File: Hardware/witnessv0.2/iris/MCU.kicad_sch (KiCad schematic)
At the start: 26 parts, among them J1 Conn_01x02, J4 Conn_01x02, U4 MCP23008-xML, U7 ESP32-C3FH4, Y1 F322540MUBCE2O

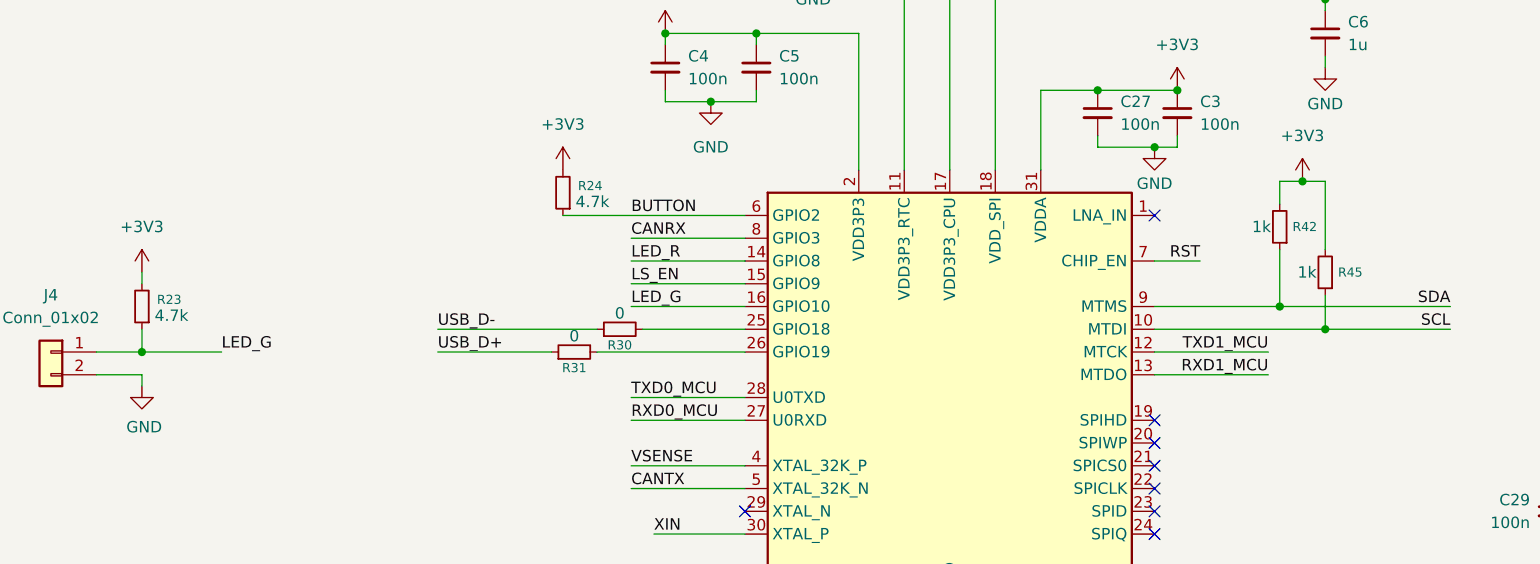
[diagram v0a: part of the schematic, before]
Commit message: iris release
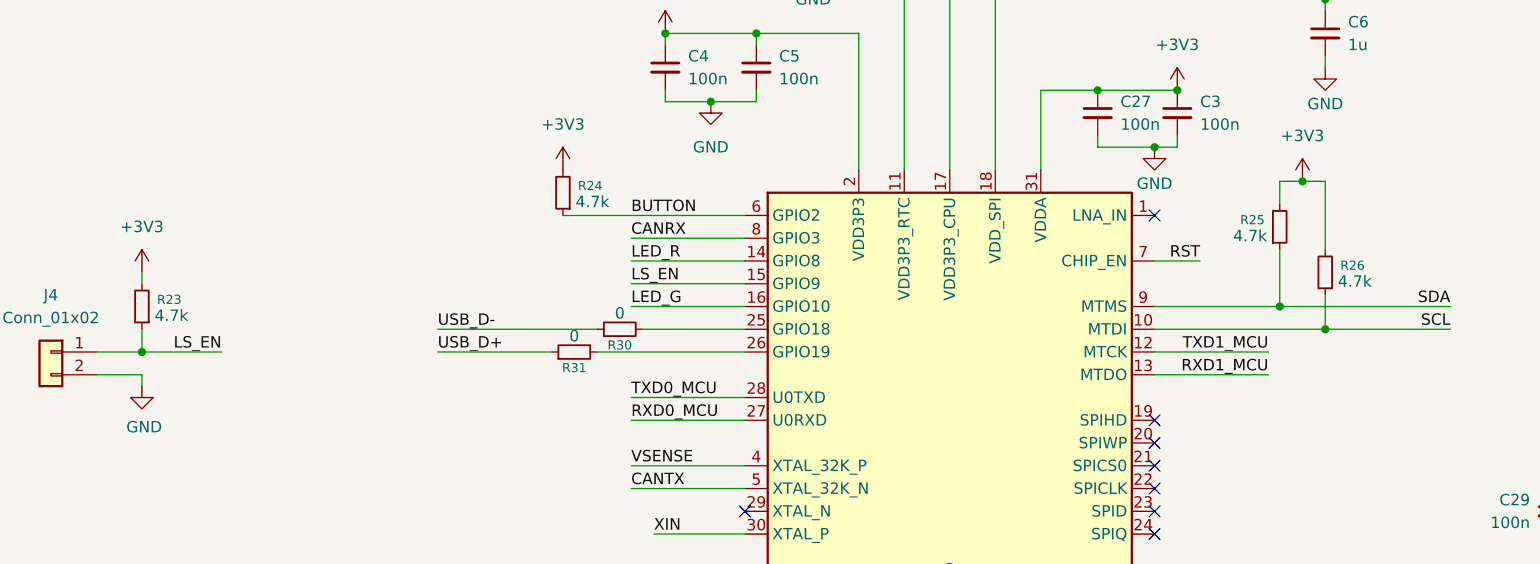
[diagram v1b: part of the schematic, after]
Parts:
- removed R42, R45: 1k, Resistor_SMD:R_0402_1005Metric, symbol Device:R_Small
- added R25, R26: 4.7k, Resistor_SMD:R_0402_1005Metric, symbol Device:R_Small
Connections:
- net +3V3: now also R25.2, R26.2
- net LED_G: no longer J4.1 (Pin_1), R23.1
- net LS_EN: now also J4.1 (Pin_1), R23.1
- net SCL: now also R26.1
- net SDA: now also R25.1
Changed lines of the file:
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@@
 		)
 	)
-	(label "LED_G"
-		(at 40.64 93.98 0)
-		(effects
-			(font
-				(size 1.27 1.27)
-			)
-			(justify left bottom)
-		)
-	)
 	(label "OUT2_EN"
 		(at 248.92 125.73 0)
@@
 		)
 	)
+	(label "LS_EN"
+		(at 40.64 93.98 180)
+		(effects
+			(font
+				(size 1.27 1.27)
+			)
+			(justify right bottom)
+		)
+	)
 	(label "USB_D-"
 		(at 245.11 22.86 0)
@@
 	)
 	(symbol
-		(lib_id "Device:R_Small")
-		(at 158.75 80.01 180)
-		(unit 1)
-		(body_style 1)
-		(exclude_from_sim no)
-		(in_bom yes)
-		(on_board yes)
-		(in_pos_files yes)
-		(dnp no)
-		(property "Reference" "R42"
-			(at 161.544 80.01 0)
-			(show_name no)
-			(do_not_autoplace no)
-			(effects
-				(font
-					(size 1.016 1.016)
-				)
-			)
-		)
-		(property "Value" "1k"
-			(at 156.718 80.01 0)
-			(show_name no)
-			(do_not_autoplace no)
-			(effects
-				(font
-					(size 1.27 1.27)
-				)
-			)
-		)
-		(property "Footprint" "Resistor_SMD:R_0402_1005Metric"
-			(at 158.75 80.01 0)
-			(hide yes)
-			(show_name no)
-			(do_not_autoplace no)
-			(effects
-				(font
-					(size 1.27 1.27)
-				)
-			)
-		)
-		(property "Datasheet" ""
-			(at 158.75 80.01 0)
-			(hide yes)
-			(show_name no)
-			(do_not_autoplace no)
-			(effects
-				(font
-					(size 1.27 1.27)
-				)
-			)
-		)
-		(property "Description" "Resistor, small symbol"
-			(at 158.75 80.01 0)
-			(hide yes)
-			(show_name no)
-			(do_not_autoplace no)
-			(effects
-				(font
-					(size 1.27 1.27)
-				)
-			)
-		)
-		(property "LCSC_Part" "C11702"
-			(at 158.75 80.01 0)
-			(hide yes)
-			(show_name no)
-			(do_not_autoplace no)
-			(effects
-				(font
-					(size 1.27 1.27)
-				)
-			)
-		)
-		(pin "2"
-		)
-		(pin "1"
-		)
-		(instances
-			(project "iris"
-				(path "/c7e4a338-55e7-4896-822a-22161197db9b/84c7cad5-6a87-4e90-b655-2e6037ab0db0"
-					(reference "R42")
-					(unit 1)
-				)
-			)
-		)
-	)
-	(symbol
 		(lib_id "power:GND")
 		(at 177.8 147.32 0)
@@
 	)
 	(symbol
-		(lib_id "Device:R_Small")
-		(at 163.83 85.09 180)
-		(unit 1)
-		(body_style 1)
-		(exclude_from_sim no)
-		(in_bom yes)
-		(on_board yes)
-		(in_pos_files yes)
-		(dnp no)
-		(property "Reference" "R45"
-			(at 166.624 85.09 0)
-			(show_name no)
-			(do_not_autoplace no)
-			(effects
-				(font
-					(size 1.016 1.016)
-				)
-			)
-		)
-		(property "Value" "1k"
-			(at 161.798 85.09 0)
-			(show_name no)
-			(do_not_autoplace no)
-			(effects
-				(font
-					(size 1.27 1.27)
-				)
-			)
-		)
-		(property "Footprint" "Resistor_SMD:R_0402_1005Metric"
-			(at 163.83 85.09 0)
-			(hide yes)
-			(show_name no)
-			(do_not_autoplace no)
-			(effects
-				(font
-					(size 1.27 1.27)
-				)
-			)
-		)
-		(property "Datasheet" ""
-			(at 163.83 85.09 0)
-			(hide yes)
-			(show_name no)
-			(do_not_autoplace no)
-			(effects
-				(font
-					(size 1.27 1.27)
-				)
-			)
-		)
-		(property "Description" "Resistor, small symbol"
-			(at 163.83 85.09 0)
-			(hide yes)
-			(show_name no)
-			(do_not_autoplace no)
-			(effects
-				(font
-					(size 1.27 1.27)
-				)
-			)
-		)
-		(property "LCSC_Part" "C11702"
-			(at 163.83 85.09 0)
-			(hide yes)
-			(show_name no)
-			(do_not_autoplace no)
-			(effects
-				(font
-					(size 1.27 1.27)
-				)
-			)
-		)
-		(pin "2"
-		)
-		(pin "1"
-		)
-		(instances
-			(project "iris"
-				(path "/c7e4a338-55e7-4896-822a-22161197db9b/84c7cad5-6a87-4e90-b655-2e6037ab0db0"
-					(reference "R45")
-					(unit 1)
-				)
-			)
-		)
-	)
-	(symbol
 		(lib_id "Device:LED_RGBA")
 		(at 156.21 168.91 0)
@@
 	)
 	(symbol
+		(lib_id "Device:R_Small")
+		(at 163.83 85.09 180)
+		(unit 1)
+		(body_style 1)
+		(exclude_from_sim no)
+		(in_bom yes)
+		(on_board yes)
+		(in_pos_files yes)
+		(dnp no)
+		(property "Reference" "R26"
+			(at 166.878 84.328 0)
+			(show_name no)
+			(do_not_autoplace no)
+			(effects
+				(font
+					(size 1.016 1.016)
+				)
+			)
+		)
+		(property "Value" "4.7k"
+			(at 167.132 86.106 0)
+			(show_name no)
+			(do_not_autoplace no)
+			(effects
+				(font
+					(size 1.27 1.27)
+				)
+			)
+		)
+		(property "Footprint" "Resistor_SMD:R_0402_1005Metric"
+			(at 163.83 85.09 0)
+			(hide yes)
+			(show_name no)
+			(do_not_autoplace no)
+			(effects
+				(font
+					(size 1.27 1.27)
+				)
+			)
+		)
+		(property "Datasheet" ""
+			(at 163.83 85.09 0)
+			(hide yes)
+			(show_name no)
+			(do_not_autoplace no)
+			(effects
+				(font
+					(size 1.27 1.27)
+				)
+			)
+		)
+		(property "Description" "Resistor, small symbol"
+			(at 163.83 85.09 0)
+			(hide yes)
+			(show_name no)
+			(do_not_autoplace no)
+			(effects
+				(font
+					(size 1.27 1.27)
+				)
+			)
+		)
+		(property "LCSC_Part" "C25900"
+			(at 163.83 85.09 0)
+			(hide yes)
+			(show_name no)
+			(do_not_autoplace no)
+			(effects
+				(font
+					(size 1.27 1.27)
+				)
+			)
+		)
+		(pin "2"
+		)
+		(pin "1"
+		)
+		(instances
+			(project "iris"
+				(path "/c7e4a338-55e7-4896-822a-22161197db9b/84c7cad5-6a87-4e90-b655-2e6037ab0db0"
+					(reference "R26")
+					(unit 1)
+				)
+			)
+		)
+	)
+	(symbol
 		(lib_id "power:GND")
 		(at 195.58 152.4 0)
@@
 					(unit 1)
 				)
+			)
+		)
+	)
+	(symbol
+		(lib_id "Device:R_Small")
+		(at 158.75 80.01 0)
+		(mirror x)
+		(unit 1)
+		(body_style 1)
+		(exclude_from_sim no)
+		(in_bom yes)
+		(on_board yes)
+		(in_pos_files yes)
+		(dnp no)
+		(property "Reference" "R25"
+			(at 155.702 79.248 0)
+			(show_name no)
+			(do_not_autoplace no)
+			(effects
+				(font
+					(size 1.016 1.016)
+				)
+			)
+		)
+		(property "Value" "4.7k"
+			(at 155.448 81.026 0)
+			(show_name no)
+			(do_not_autoplace no)
+			(effects
+				(font
+					(size 1.27 1.27)
+				)
+			)
+		)
+		(property "Footprint" "Resistor_SMD:R_0402_1005Metric"
+			(at 158.75 80.01 0)
+			(hide yes)
+			(show_name no)
+			(do_not_autoplace no)
+			(effects
+				(font
+					(size 1.27 1.27)
+				)
+			)
+		)
+		(property "Datasheet" ""
+			(at 158.75 80.01 0)
+			(hide yes)
+			(show_name no)
+			(do_not_autoplace no)
+			(effects
+				(font
+					(size 1.27 1.27)
+				)
+			)
+		)
+		(property "Description" "Resistor, small symbol"
+			(at 158.75 80.01 0)
+			(hide yes)
+			(show_name no)
+			(do_not_autoplace no)
+			(effects
+				(font
+					(size 1.27 1.27)
+				)
+			)
+		)
+		(property "LCSC_Part" "C25900"
+			(at 158.75 80.01 0)
+			(hide yes)
+			(show_name no)
+			(do_not_autoplace no)
+			(effects
+				(font
+					(size 1.27 1.27)
+				)
+			)
+		)
+		(pin "2"
+		)
+		(pin "1"
+		)
+		(instances
+			(project "iris"
+				(path "/c7e4a338-55e7-4896-822a-22161197db9b/84c7cad5-6a87-4e90-b655-2e6037ab0db0"
+					(reference "R25")
+					(unit 1)
+				)
